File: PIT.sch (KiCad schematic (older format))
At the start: 1 part, among them U6 82C54

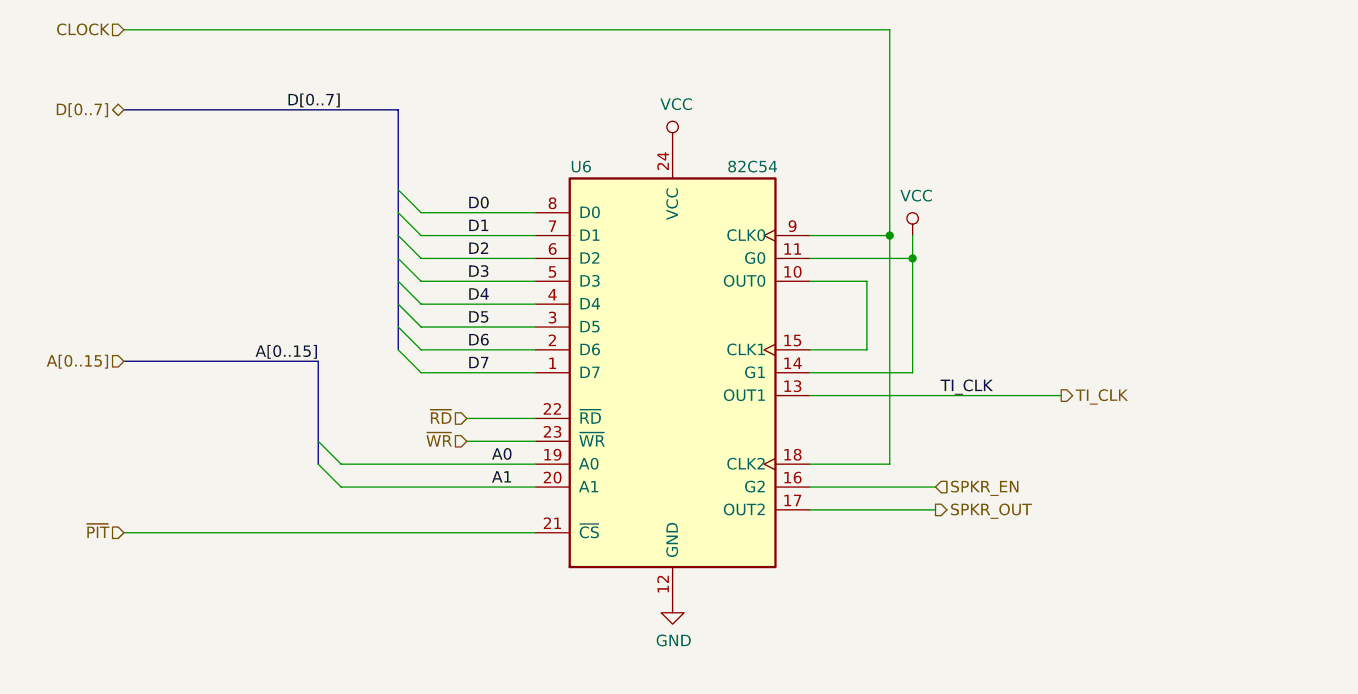
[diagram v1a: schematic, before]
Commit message: RevC
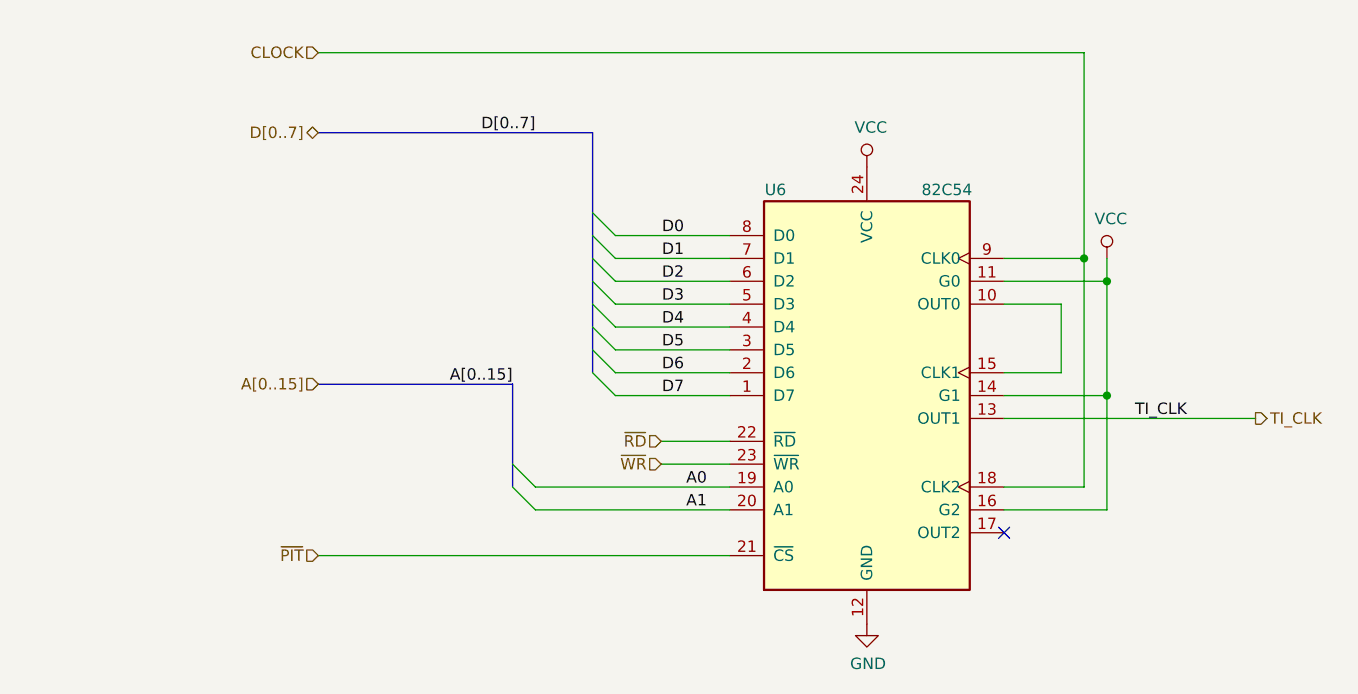
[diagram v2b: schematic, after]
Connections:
- net SPKR_EN is gone; now on net VCC: U6.16 (G2)
- net SPKR_OUT: no longer names the net of U6.17 (OUT2)
- no-connect marks 0 -> 1
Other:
- moved on the sheet: U6
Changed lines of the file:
@@
 EELAYER 30 0
 EELAYER END
-$Descr A4 11693 8268
+$Descr USLetter 11000 8500
 encoding utf-8
 Sheet 4 6
 Title "PIT / SOUND"
-Date "2018-09-17"
-Rev "A"
+Date "2018-09-27"
+Rev "C"
 Comp ""
 Comment1 ""
@@
 L Timer:82C54 U6
 U 1 1 5B98D78A
-P 3550 3000
-F 0 "U6" H 3150 3900 50  0000 C CNN
-F 1 "82C54" H 3900 3900 50  0000 C CNN
-F 2 "Package_DIP:DIP-24_W15.24mm_Socket" H 3600 3250 50  0001 C CNN
-F 3 "http://download.intel.com/design/archives/periphrl/docs/23124406.pdf" H 3100 3900 50  0001 C CNN
-	1    3550 3000
+P 4400 3100
+F 0 "U6" H 4000 4000 50  0000 C CNN
+F 1 "82C54" H 4750 4000 50  0000 C CNN
+F 2 "Package_DIP:DIP-24_W15.24mm_Socket" H 4450 3350 50  0001 C CNN
+F 3 "http://download.intel.com/design/archives/periphrl/docs/23124406.pdf" H 3950 4000 50  0001 C CNN
+	1    4400 3100
 	1    0    0    -1
 $EndComp
@@
 L power:GND #PWR014
 U 1 1 5B98D8C0
-P 3550 4000
-F 0 "#PWR014" H 3550 3750 50  0001 C CNN
-F 1 "GND" H 3555 3827 50  0000 C CNN
-F 2 "" H 3550 4000 50  0001 C CNN
-F 3 "" H 3550 4000 50  0001 C CNN
-	1    3550 4000
+P 4400 4100
+F 0 "#PWR014" H 4400 3850 50  0001 C CNN
+F 1 "GND" H 4405 3927 50  0000 C CNN
+F 2 "" H 4400 4100 50  0001 C CNN
+F 3 "" H 4400 4100 50  0001 C CNN
+	1    4400 4100
 	1    0    0    -1
 $EndComp
@@
 L power:VCC #PWR013
 U 1 1 5B98D900
-P 3550 2000
-F 0 "#PWR013" H 3550 1850 50  0001 C CNN
-F 1 "VCC" H 3567 2173 50  0000 C CNN
-F 2 "" H 3550 2000 50  0001 C CNN
-F 3 "" H 3550 2000 50  0001 C CNN
-	1    3550 2000
+P 4400 2100
+F 0 "#PWR013" H 4400 1950 50  0001 C CNN
+F 1 "VCC" H 4417 2273 50  0000 C CNN
+F 2 "" H 4400 2100 50  0001 C CNN
+F 3 "" H 4400 2100 50  0001 C CNN
+	1    4400 2100
 	1    0    0    -1
 $EndComp
-Text HLabel 1150 1850 0    50   BiDi ~ 0
+Text HLabel 2000 1950 0    50   BiDi ~ 0
 D[0..7]
-Text HLabel 1150 2950 0    50   Input ~ 0
+Text HLabel 2000 3050 0    50   Input ~ 0
 A[0..15]
-Text HLabel 2650 3200 0    50   Input ~ 0
+Text HLabel 3500 3300 0    50   Input ~ 0
 ~RD
-Text HLabel 2650 3300 0    50   Input ~ 0
+Text HLabel 3500 3400 0    50   Input ~ 0
 ~WR
 Entry Wire Line
-	2000 3300 2100 3400
+	2850 3400 2950 3500
 Entry Wire Line
-	2000 3400 2100 3500
+	2850 3500 2950 3600
 Wire Wire Line
-	2650 3200 2950 3200
+	3500 3300 3800 3300
 Wire Wire Line
-	2950 3300 2650 3300
+	3800 3400 3500 3400
 Wire Wire Line
-	2950 3400 2100 3400
+	3800 3500 2950 3500
 Wire Wire Line
-	2100 3500 2950 3500
-Text Label 2850 3400 2    50   ~ 0
+	2950 3600 3800 3600
+Text Label 3700 3500 2    50   ~ 0
 A0
-Text Label 2850 3500 2    50   ~ 0
+Text Label 3700 3600 2    50   ~ 0
 A1
 Wire Bus Line
-	1150 2950 2000 2950
-Text Label 2000 2950 2    50   ~ 0
+	2000 3050 2850 3050
+Text Label 2850 3050 2    50   ~ 0
 A[0..15]
 Entry Wire Line
-	2350 2900 2450 3000
+	3200 3000 3300 3100
 Entry Wire Line
-	2350 2800 2450 2900
+	3200 2900 3300 3000
 Entry Wire Line
-	2350 2700 2450 2800
+	3200 2800 3300 2900
 Entry Wire Line
-	2350 2600 2450 2700
+	3200 2700 3300 2800
 Entry Wire Line
-	2350 2500 2450 2600
+	3200 2600 3300 2700
 Entry Wire Line
-	2350 2400 2450 2500
+	3200 2500 3300 2600
 Entry Wire Line
-	2350 2300 2450 2400
+	3200 2400 3300 2500
 Entry Wire Line
-	2350 2200 2450 2300
+	3200 2300 3300 2400
 Wire Bus Line
-	2350 1850 1150 1850
+	3200 1950 2000 1950
 Wire Wire Line
-	2450 2300 2950 2300
+	3300 2400 3800 2400
 Wire Wire Line
-	2950 2400 2450 2400
+	3800 2500 3300 2500
 Wire Wire Line
-	2450 2500 2950 2500
+	3300 2600 3800 2600
 Wire Wire Line
-	2950 2600 2450 2600
+	3800 2700 3300 2700
 Wire Wire Line
-	2950 2700 2450 2700
+	3800 2800 3300 2800
 Wire Wire Line
-	2950 2800 2450 2800
+	3800 2900 3300 2900
 Wire Wire Line
-	2950 2900 2450 2900
+	3800 3000 3300 3000
 Wire Wire Line
-	2950 3000 2450 3000
-Text Label 2100 1850 2    50   ~ 0
+	3800 3100 3300 3100
+Text Label 2950 1950 2    50   ~ 0
 D[0..7]
-Text Label 2750 2300 2    50   ~ 0
+Text Label 3600 2400 2    50   ~ 0
 D0
-Text Label 2750 2400 2    50   ~ 0
+Text Label 3600 2500 2    50   ~ 0
 D1
-Text Label 2750 2500 2    50   ~ 0
+Text Label 3600 2600 2    50   ~ 0
 D2
-Text Label 2750 2600 2    50   ~ 0
+Text Label 3600 2700 2    50   ~ 0
 D3
-Text Label 2750 2700 2    50   ~ 0
+Text Label 3600 2800 2    50   ~ 0
 D4
-Text Label 2750 2800 2    50   ~ 0
+Text Label 3600 2900 2    50   ~ 0
 D5
-Text Label 2750 2900 2    50   ~ 0
+Text Label 3600 3000 2    50   ~ 0
 D6
-Text Label 2750 3000 2    50   ~ 0
+Text Label 3600 3100 2    50   ~ 0
 D7
-Text HLabel 1150 1500 0    50   Input ~ 0
+Text HLabel 2000 1600 0    50   Input ~ 0
 CLOCK
 Wire Wire Line
-	1150 1500 4500 1500
+	2000 1600 5350 1600
 Wire Wire Line
-	4500 1500 4500 2400
+	5350 1600 5350 2500
 Wire Wire Line
-	4150 2900 4400 2900
+	5000 3000 5250 3000
 Wire Wire Line
-	4150 2400 4500 2400
-Text HLabel 1150 3700 0    50   Input ~ 0
+	5000 2500 5350 2500
+Text HLabel 2000 3800 0    50   Input ~ 0
 ~PIT
 Wire Wire Line
-	2950 3700 1150 3700
+	3800 3800 2000 3800
 Wire Wire Line
-	4150 2600 4400 2600
+	5000 2700 5250 2700
 Wire Wire Line
-	4400 2600 4400 2900
+	5250 2700 5250 3000
 $Comp
 L power:VCC #PWR015
 U 1 1 5BBB10AA
-P 4600 2400
-F 0 "#PWR015" H 4600 2250 50  0001 C CNN
-F 1 "VCC" H 4617 2573 50  0000 C CNN
-F 2 "" H 4600 2400 50  0001 C CNN
-F 3 "" H 4600 2400 50  0001 C CNN
-	1    4600 2400
+P 5450 2500
+F 0 "#PWR015" H 5450 2350 50  0001 C CNN
+F 1 "VCC" H 5467 2673 50  0000 C CNN
+F 2 "" H 5450 2500 50  0001 C CNN
+F 3 "" H 5450 2500 50  0001 C CNN
+	1    5450 2500
 	1    0    0    -1
 $EndComp
 Wire Wire Line
-	4150 2500 4600 2500
+	5000 2600 5450 2600
 Wire Wire Line
-	4600 2500 4600 2400
+	5450 2600 5450 2500
 Wire Wire Line
-	4150 3000 4600 3000
+	5000 3100 5450 3100
 Wire Wire Line
-	4600 3000 4600 2500
-Connection ~ 4600 2500
+	5450 3100 5450 2600
+Connection ~ 5450 2600
 Wire Wire Line
-	4150 3100 5250 3100
-Text Label 4950 3100 2    50   ~ 0
+	5000 3200 6100 3200
+Text Label 5800 3200 2    50   ~ 0
 TI_CLK
-Text HLabel 5250 3100 2    50   Output ~ 0
+Text HLabel 6100 3200 2    50   Output ~ 0
 TI_CLK
-Text HLabel 4700 3500 2    50   Input ~ 0
-SPKR_EN
 Wire Wire Line
-	4700 3500 4150 3500
-Text HLabel 4700 3600 2    50   Output ~ 0
-SPKR_OUT
+	5000 3500 5350 3500
 Wire Wire Line
-	4150 3400 4500 3400
+	5350 3500 5350 2500
+Connection ~ 5350 2500
 Wire Wire Line
-	4500 3400 4500 2400
-Connection ~ 4500 2400
+	5000 3600 5450 3600
 Wire Wire Line
-	4700 3600 4150 3600
+	5450 3600 5450 3100
+Connection ~ 5450 3100
+NoConn ~ 5000 3700
 Wire Bus Line
-	2000 2950 2000 3400
+	2850 3050 2850 3500
 Wire Bus Line
-	2350 1850 2350 2900
+	3200 1950 3200 3000
 $EndSCHEMATC
